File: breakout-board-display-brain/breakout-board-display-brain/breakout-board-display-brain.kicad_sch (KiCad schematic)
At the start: 7 parts, among them J1 Conn_01x15_Socket, J2 Conn_01x15_Socket, J3 Conn_01x16_Female, J4 Conn_01x02_Socket, SW1 RotaryEncoder_Switch

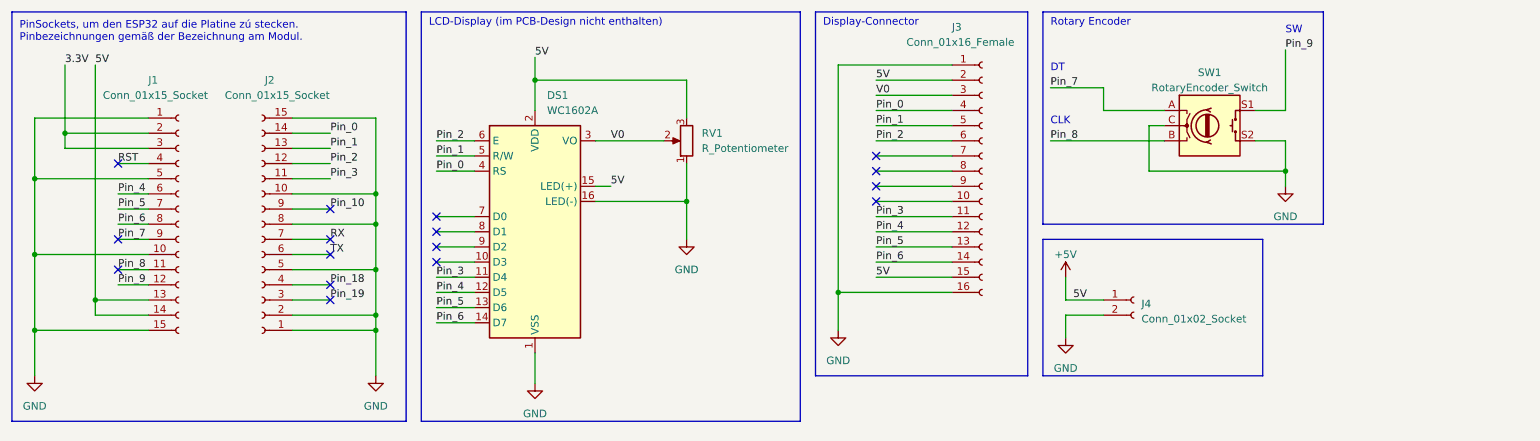
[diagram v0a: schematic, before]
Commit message: ...
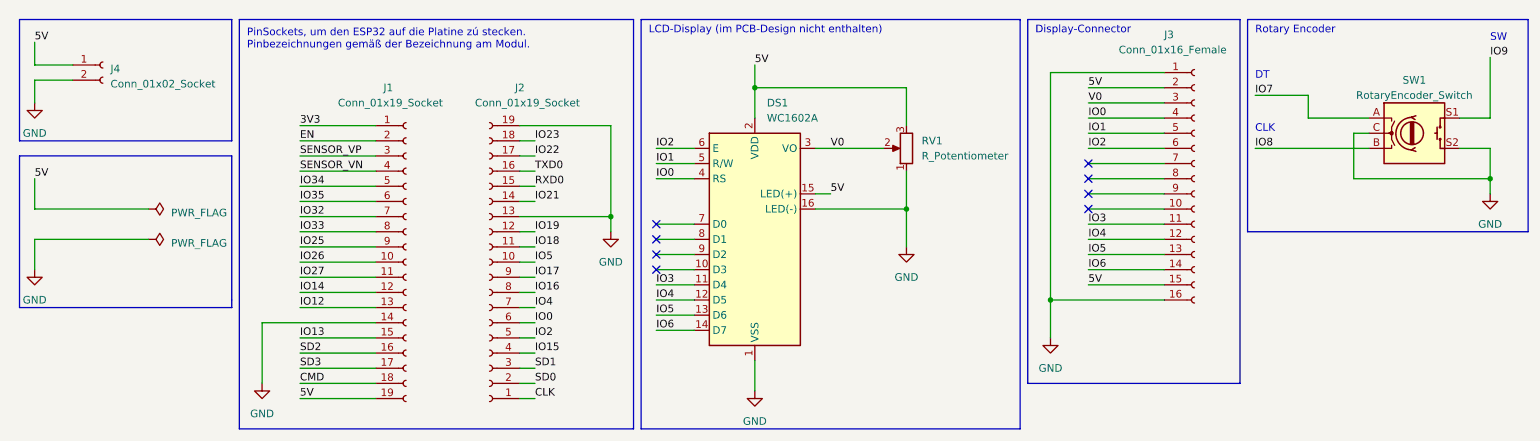
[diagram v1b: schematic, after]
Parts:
- removed J1, J2: Conn_01x15_Socket, Connector_PinSocket_2.54mm:PinSocket_1x15_P2.54mm_Vertical, symbol Connector:Conn_01x15_Socket
- added J1, J2: Conn_01x19_Socket, Connector_PinSocket_2.54mm:PinSocket_1x19_P2.54mm_Vertical, symbol Connector:Conn_01x19_Socket
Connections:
- net GND: now also J1.14 (Pin_14), J2.13 (Pin_13), J2.19 (Pin_19)
- net +5V renamed 5V
- net 5V: now also J1.19 (Pin_19)
- net Pin_0 renamed IO0
- net IO0: now also J2.6 (Pin_6)
- net Pin_1 renamed IO1
- net Pin_2 renamed IO2
- net IO2: now also J2.5 (Pin_5)
- net Pin_3 renamed IO3
- net Pin_4 renamed IO4
- net IO4: now also J2.7 (Pin_7)
- net Pin_5 renamed IO5
- net IO5: now also J2.10 (Pin_10)
- net Pin_6 renamed IO6
- net Pin_7 renamed IO7
- net Pin_8 renamed IO8
- net Pin_9 renamed IO9
- new net 3V3: J1.1 (Pin_1)
- new net CLK: J2.1 (Pin_1)
- new net CMD: J1.18 (Pin_18)
- new net EN: J1.2 (Pin_2)
- new net IO12: J1.13 (Pin_13)
- new net IO13: J1.15 (Pin_15)
- new net IO14: J1.12 (Pin_12)
- new net IO15: J2.4 (Pin_4)
- new net IO16: J2.8 (Pin_8)
- new net IO17: J2.9 (Pin_9)
- new net IO18: J2.11 (Pin_11)
- new net IO19: J2.12 (Pin_12)
- new net IO21: J2.14 (Pin_14)
- new net IO22: J2.17 (Pin_17)
- new net IO23: J2.18 (Pin_18)
- new net IO25: J1.9 (Pin_9)
- new net IO26: J1.10 (Pin_10)
- new net IO27: J1.11 (Pin_11)
- new net IO32: J1.7 (Pin_7)
- new net IO33: J1.8 (Pin_8)
- new net IO34: J1.5 (Pin_5)
- new net IO35: J1.6 (Pin_6)
- new net RXD0: J2.15 (Pin_15)
- new net SD0: J2.2 (Pin_2)
- new net SD1: J2.3 (Pin_3)
- new net SD2: J1.16 (Pin_16)
- new net SD3: J1.17 (Pin_17)
- new net SENSOR_VN: J1.4 (Pin_4)
- new net SENSOR_VP: J1.3 (Pin_3)
- new net TXD0: J2.16 (Pin_16)
- no-connect marks 16 -> 8
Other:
- moved on the sheet: DS1, J3, J4, RV1, SW1
